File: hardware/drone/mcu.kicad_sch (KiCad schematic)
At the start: 35 parts, among them J3 USB_C_Receptacle_USB2.0_16P, J4 Conn_ARM_SWD_TagConnect_TC2030, SW1 SW_MEC_5E, U1 STM32N645I0, U20 TVS0500DRV, U6 MX25UW25645GXDI00, Y3 Crystal_GND24

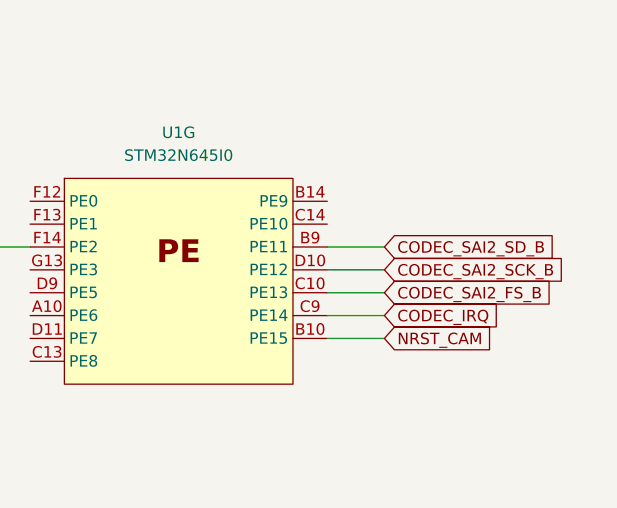
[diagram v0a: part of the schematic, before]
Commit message: Small cleanup
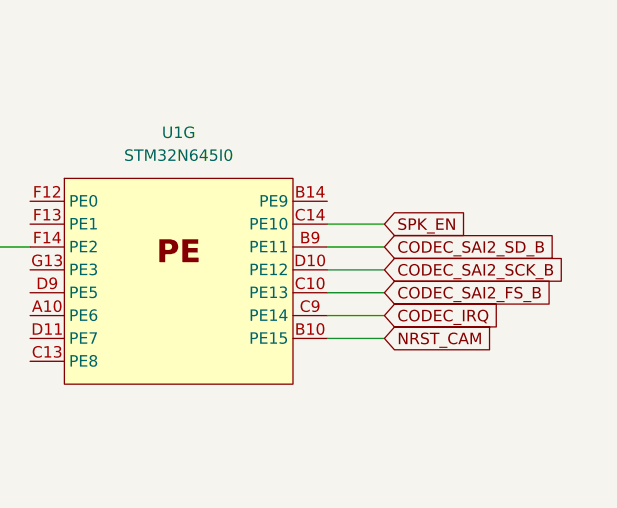
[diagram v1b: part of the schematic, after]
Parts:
- R25, R26, R27, R28, R29: footprint BM08BSRSSTBLFSN -> (none)
- U1: footprint (none) -> STM32N645I0:BGA178C80P14X14_1200X1200X100
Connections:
- net SPK_EN: now reaches U1.C14 (PE10)
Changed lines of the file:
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@@
 	(wire
 		(pts
+			(xy 537.21 46.99) (xy 543.56 46.99)
+		)
+		(stroke
+			(width 0)
+			(type default)
+		)
+	)
+	(wire
+		(pts
 			(xy 200.66 50.8) (xy 204.47 50.8)
 		)
@@
 			3.81 3.81 3.81 3.81 3.81 3.81 3.81 3.81 3.81 3.81 3.81 3.81 3.81 3.81
 			3.81 3.81 3.81 3.81 3.81 3.81 3.81 3.81 3.81 3.81 3.81 3.81 3.81 3.81
-			3.81 3.81 3.81 3.81 3.81 3.81 3.81
+			3.81 3.81 3.81 3.81 3.81 3.81 3.81 3.81
 		)
 		(cells
@@
 				)
 			)
+			(table_cell "C14"
+				(exclude_from_sim no)
+				(at 382.905 367.665 0)
+				(size 20.32 3.81)
+				(margins 0.9525 0.9525 0.9525 0.9525)
+				(span 1 1)
+				(fill
+					(type none)
+				)
+				(effects
+					(font
+						(size 2.032 2.032)
+					)
+					(justify left top)
+				)
+			)
+			(table_cell "PE10"
+				(exclude_from_sim no)
+				(at 403.225 367.665 0)
+				(size 20.32 3.81)
+				(margins 0.9525 0.9525 0.9525 0.9525)
+				(span 1 1)
+				(fill
+					(type none)
+				)
+				(effects
+					(font
+						(size 2.032 2.032)
+					)
+					(justify left top)
+				)
+			)
+			(table_cell "GPIO (SPK_EN)"
+				(exclude_from_sim no)
+				(at 423.545 367.665 0)
+				(size 40.64 3.81)
+				(margins 0.9525 0.9525 0.9525 0.9525)
+				(span 1 1)
+				(fill
+					(type none)
+				)
+				(effects
+					(font
+						(size 2.032 2.032)
+					)
+					(justify left top)
+				)
+			)
+			(table_cell "Speaker Amp"
+				(exclude_from_sim no)
+				(at 464.185 367.665 0)
+				(size 38.1 3.81)
+				(margins 0.9525 0.9525 0.9525 0.9525)
+				(span 1 1)
+				(fill
+					(type none)
+				)
+				(effects
+					(font
+						(size 2.032 2.032)
+					)
+					(justify left top)
+				)
+			)
+			(table_cell ""
+				(exclude_from_sim no)
+				(at 502.285 367.665 0)
+				(size 38.1 3.81)
+				(margins 0.9525 0.9525 0.9525 0.9525)
+				(span 1 1)
+				(fill
+					(type none)
+				)
+				(effects
+					(font
+						(size 2.032 2.032)
+					)
+					(justify left top)
+				)
+			)
 		)
 	)
@@
 		)
 	)
+	(global_label "SPK_EN"
+		(shape input)
+		(at 543.56 46.99 0)
+		(fields_autoplaced yes)
+		(effects
+			(font
+				(size 1.27 1.27)
+			)
+			(justify left)
+		)
+		(property "Intersheetrefs" "${INTERSHEET_REFS}"
+			(at 553.7418 46.99 0)
+			(hide yes)
+			(show_name no)
+			(do_not_autoplace no)
+			(effects
+				(font
+					(size 1.27 1.27)
+				)
+				(justify left)
+			)
+		)
+	)
 	(global_label "IMU_INT1"
 		(shape input)
@@
 			)
 		)
-		(property "Footprint" "BM08BSRSSTBLFSN"
+		(property "Footprint" ""
 			(at 202.438 57.15 90)
 			(hide yes)
@@
 			)
 		)
-		(property "Footprint" ""
+		(property "Footprint" "STM32N645I0:BGA178C80P14X14_1200X1200X100"
 			(at 55.88 54.61 0)
 			(hide yes)
@@
 			)
 		)
-		(property "Footprint" "BM08BSRSSTBLFSN"
+		(property "Footprint" ""
 			(at 219.71 52.578 90)
 			(hide yes)
@@
 			)
 		)
-		(property "Footprint" ""
+		(property "Footprint" "STM32N645I0:BGA178C80P14X14_1200X1200X100"
 			(at 448.31 54.61 0)
 			(hide yes)
@@
 			)
 		)
-		(property "Footprint" ""
+		(property "Footprint" "STM32N645I0:BGA178C80P14X14_1200X1200X100"
 			(at 173.99 209.55 0)
 			(hide yes)
@@
 			)
 		)
-		(property "Footprint" ""
+		(property "Footprint" "STM32N645I0:BGA178C80P14X14_1200X1200X100"
 			(at 419.1 101.6 0)
 			(hide yes)
@@
 			)
 		)
-		(property "Footprint" ""
+		(property "Footprint" "STM32N645I0:BGA178C80P14X14_1200X1200X100"
 			(at 327.66 46.99 0)
 			(hide yes)
@@
 			)
 		)
-		(property "Footprint" ""
+		(property "Footprint" "STM32N645I0:BGA178C80P14X14_1200X1200X100"
 			(at 520.7 53.34 0)
 			(hide yes)
@@
 			)
 		)
-		(property "Footprint" "BM08BSRSSTBLFSN"
+		(property "Footprint" ""
 			(at 306.07 187.198 90)
 			(hide yes)
@@
 			)
 		)
-		(property "Footprint" ""
+		(property "Footprint" "STM32N645I0:BGA178C80P14X14_1200X1200X100"
 			(at 152.4 50.8 0)
 			(hide yes)
@@
 			)
 		)
-		(property "Footprint" "BM08BSRSSTBLFSN"
+		(property "Footprint" ""
 			(at 306.07 189.738 90)
 			(hide yes)
@@
 			)
 		)
-		(property "Footprint" ""
+		(property "Footprint" "STM32N645I0:BGA178C80P14X14_1200X1200X100"
 			(at 196.85 97.79 0)
 			(hide yes)
@@
 			)
 		)
-		(property "Footprint" ""
+		(property "Footprint" "STM32N645I0:BGA178C80P14X14_1200X1200X100"
 			(at 320.04 92.71 0)
 			(hide yes)
@@
 			)
 		)
-		(property "Footprint" "BM08BSRSSTBLFSN"
+		(property "Footprint" ""
 			(at 208.28 52.578 90)
 			(hide yes)
@@
 			)
 		)
-		(property "Footprint" ""
+		(property "Footprint" "STM32N645I0:BGA178C80P14X14_1200X1200X100"
 			(at 120.65 115.57 0)
 			(hide yes)
@@
 			)
 		)
-		(property "Footprint" ""
+		(property "Footprint" "STM32N645I0:BGA178C80P14X14_1200X1200X100"
 			(at 237.49 210.82 0)
 			(hide yes)
